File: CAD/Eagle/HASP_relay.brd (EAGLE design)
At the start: 42.6 x 36.1 mm, 15 parts

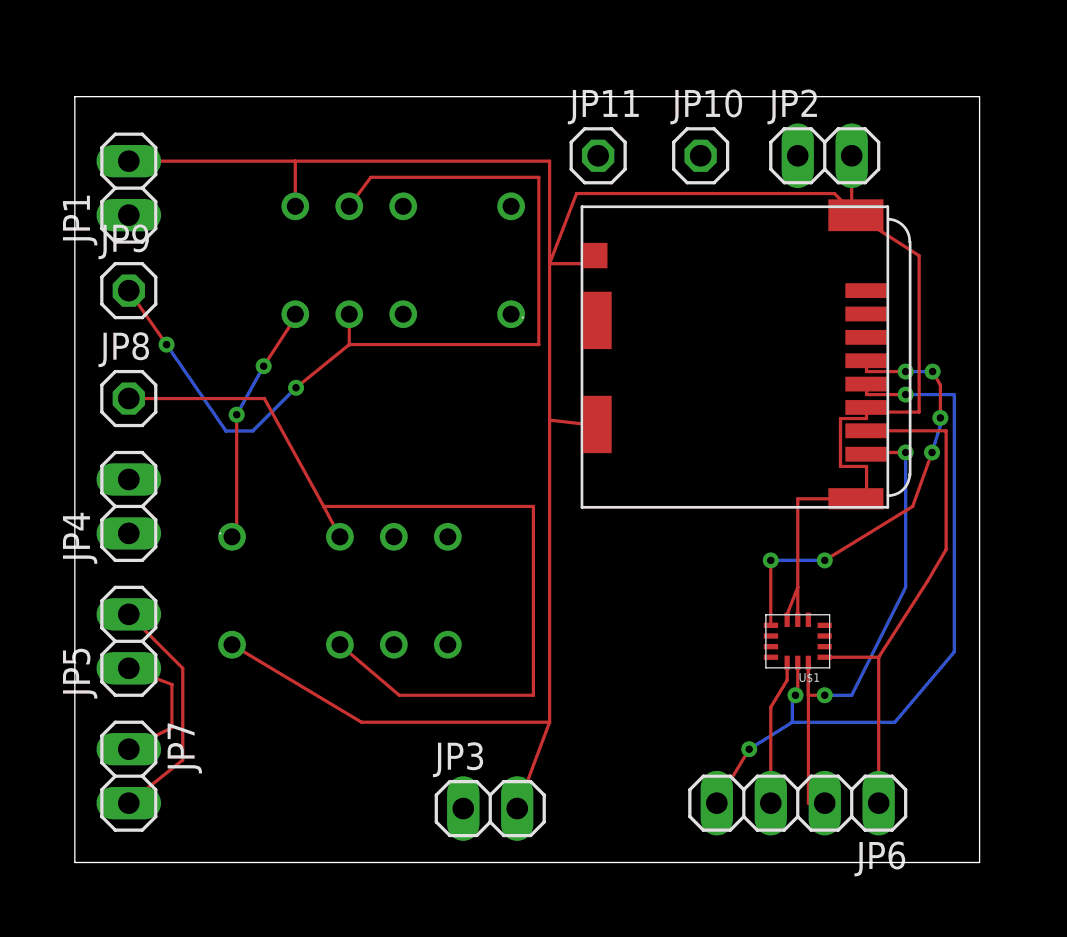
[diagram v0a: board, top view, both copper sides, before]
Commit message: Relay board
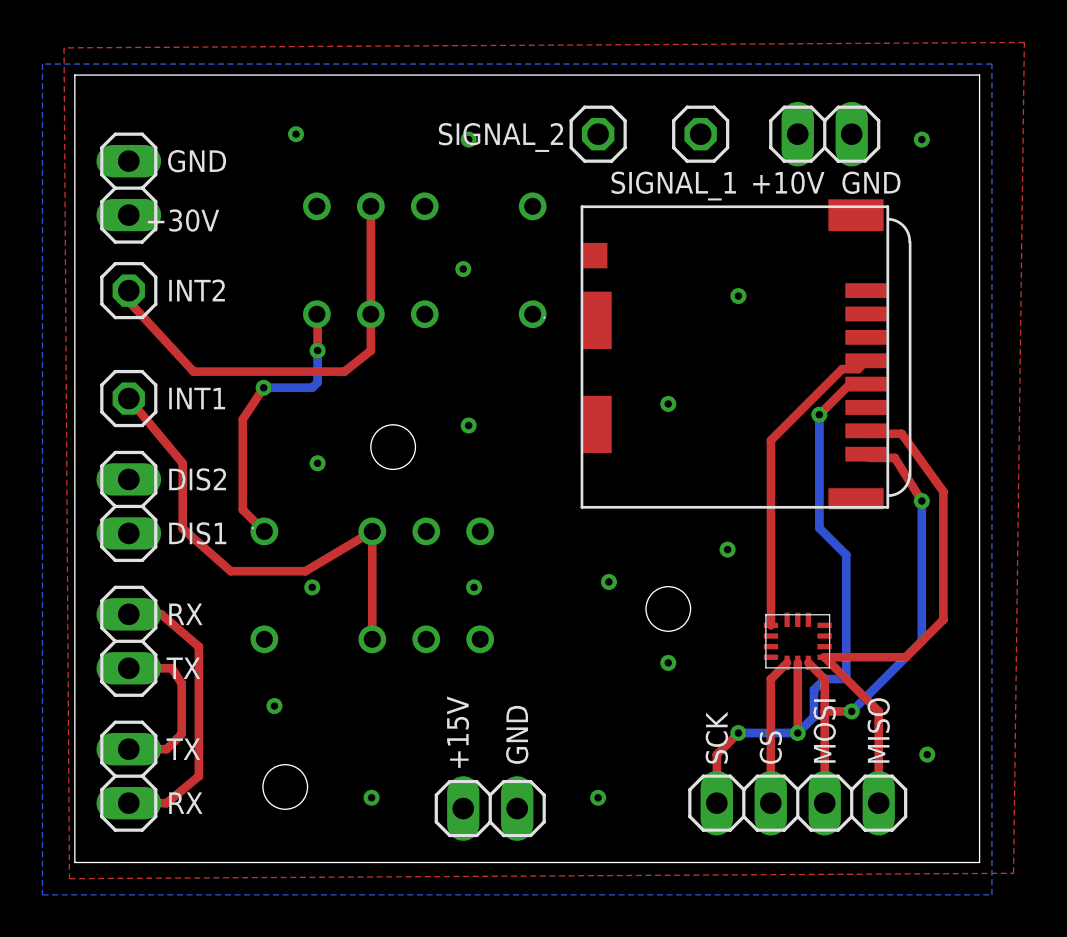
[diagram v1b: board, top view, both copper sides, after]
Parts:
- moved U$2 1.55 mm to (7.87, 9.40)
- moved U$3 1.02 mm to (22.6, 32.0)
- moved JP10 1.02 mm to (29.5, 34.3)
- moved JP11 1.02 mm to (24.6, 34.3)
- moved JP2 1.02 mm to (35.3, 34.3)
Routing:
- net GND: track 124.2 -> 1.39 mm, vias 0 -> 16
- net INT2: track 43.2 -> 20.5 mm, vias 2 -> 0
- net INT1: track 42.6 -> 22.3 mm
- net +3V3: track 20.8 -> 14.8 mm, vias 6 -> 0
- net SCK: track 34.3 -> 29.7 mm
- net RX: track 11.2 -> 13.7 mm
- net PWR: track 11.5 -> 13.4 mm
- net TX: track 6.47 -> 8.05 mm
- net MOSI: track 24.9 -> 23.7 mm
- net MISO: track 24.7 -> 25.4 mm
- added copper zone on layer 1, net GND
- added copper zone on layer 16, net GND
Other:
- board size 42.6 x 36.1 mm -> 42.6 x 37.1 mm
- board text added: "+10V"
- board text added: "+15V"
- board text added: "+30V"
- board text added: "CS"
- board text added: "DIS1"
- board text added: "DIS2"
- board text added: "GND"
- board text added: "INT1"
- board text added: "INT2"
- board text added: "MISO"
- board text added: "MOSI"
- board text added: "RX"
- board text added: "SCK"
- board text added: "SIGNAL_1"
- board text added: "SIGNAL_2"
- board text added: "TX"
